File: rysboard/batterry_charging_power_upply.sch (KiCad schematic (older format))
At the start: 28 parts, among them J20 Conn_01x02, Q5 DMP3036SSD-13, Q6 DMP3036SSD-13, Q7 NST847BDP6T5G, Q9 Si7938DP-T1-GE3, U12 LTC4007

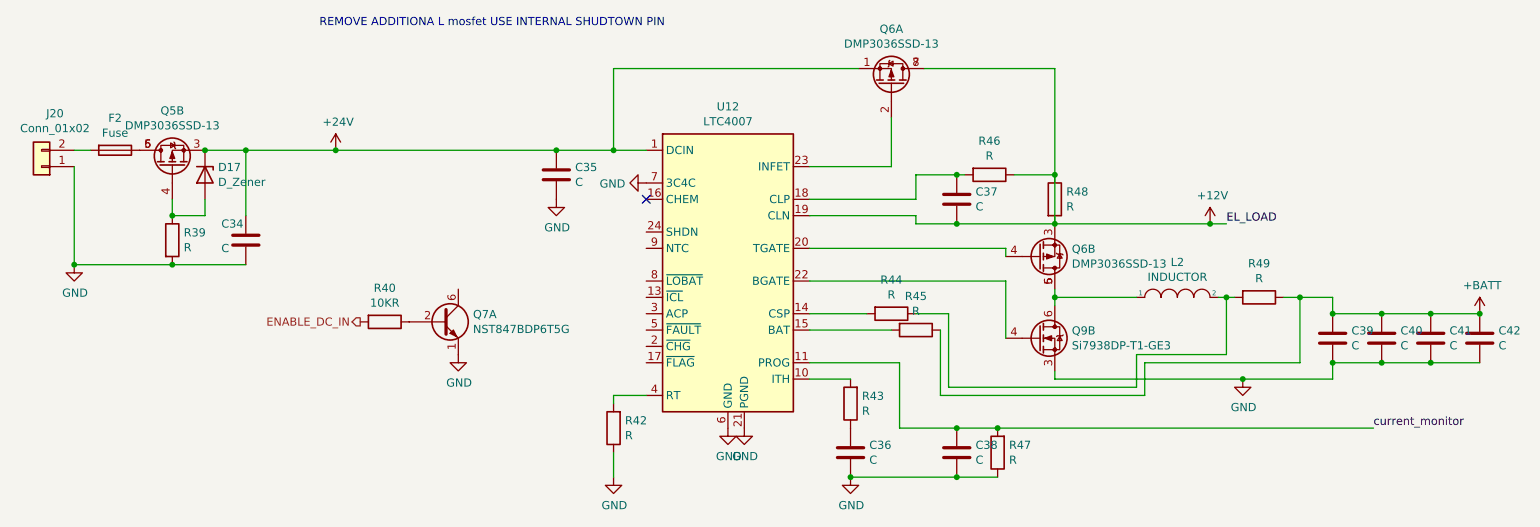
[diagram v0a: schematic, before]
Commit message: more work done
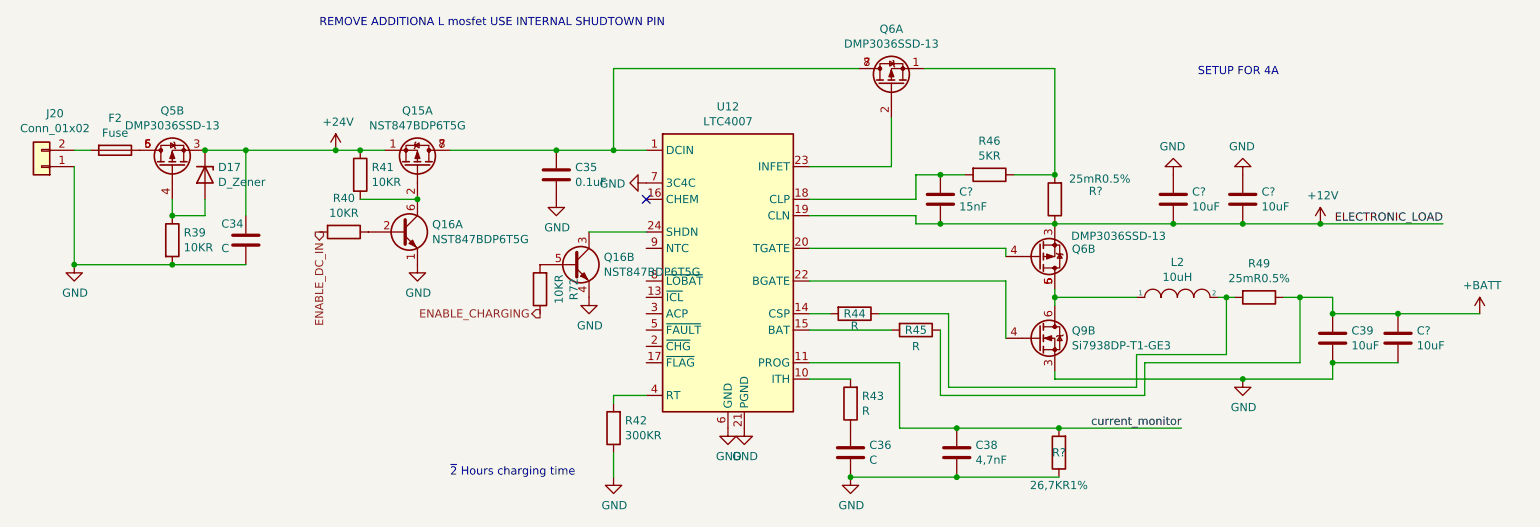
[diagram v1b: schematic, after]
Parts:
- removed C37, C40, C41, C42: C, symbol Device:C
- removed Q7: NST847BDP6T5G, Package_TO_SOT_SMD:SOT-963, symbol rysboard:NST847BDP6T5G
- removed R47, R48: R, symbol Device:R
- added C?: 15nF, Capacitor_SMD:C_0603_1608Metric, symbol Device:C
- added C? (x3): 10uF, Capacitor_SMD:C_1206_3216Metric, symbol Device:C
- added Q15: NST847BDP6T5G, Package_TO_SOT_SMD:SOT-963, symbol rysboard:DMP3036SSD-13
- added Q16: NST847BDP6T5G, Package_TO_SOT_SMD:SOT-963, symbol rysboard:NST847BDP6T5G
- added R41: 10KR, Resistor_SMD:R_0603_1608Metric_Pad1.05x0.95mm_HandSolder, symbol Device:R
- added R72: 10KR, Resistor_SMD:R_0603_1608Metric, symbol Device:R
- added R?: 26,7KR1%, Resistor_SMD:R_0603_1608Metric, symbol Device:R
- added R?: 25mR0.5%, symbol Device:R
- C35: value C -> 0.1uF; footprint (none) -> Capacitor_SMD:C_0603_1608Metric
- C38: value C -> 4,7nF; footprint (none) -> Capacitor_SMD:C_0603_1608Metric_Pad1.05x0.95mm_HandSolder
- C39: value C -> 10uF; footprint (none) -> Capacitor_SMD:C_1206_3216Metric
- L2: value INDUCTOR -> 10uH
- R39: value R -> 10KR; footprint (none) -> Resistor_SMD:R_0603_1608Metric_Pad1.05x0.95mm_HandSolder
- R42: value R -> 300KR; footprint (none) -> Resistor_SMD:R_0603_1608Metric_Pad1.05x0.95mm_HandSolder
- R46: value R -> 5KR; footprint (none) -> Resistor_SMD:R_0603_1608Metric_Pad1.05x0.95mm_HandSolder
- R49: value R -> 25mR0.5%
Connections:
- net +12V: now also C?.2, C?.2, C?.2, R?.1; no longer Q6.7 (d), Q6.8 (d), R46.1
- net +24V: now also Q15.1 (S1), R41.1; no longer C35.1, Q6.1 (S1), U12.1 (DCIN)
- net +BATT: now also C?.1
- net GND: now also C?.1, C?.1, C?.2, Q16.1 (E1), Q16.4 (E2), R?.1
- net current_monitor: now also R?.2
- net at R46.2, U12.18 (CLP): now also C?.1
- net at U12.24 (SHDN): now also Q16.3 (C2)
- net at R40.1: now also Q16.2 (B1)
- new net: C35.1, Q15.7 (d), Q15.8 (d), Q6.7 (d), Q6.8 (d), U12.1 (DCIN)
- new net: Q6.1 (S1), R46.1, R?.2
- new net: Q15.2 (G1), Q16.6 (C1), R41.2
- new net: Q16.5 (B2), R72.2
- new net ENABLE_CHARGING: R72.1
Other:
- note added: "SETUP FOR 4A"
- note added: "~2 Hours charging time"
- moved on the sheet: R40, R44
